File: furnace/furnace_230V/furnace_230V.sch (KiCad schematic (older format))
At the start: 3 parts

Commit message: Add files via upload
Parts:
- removed J?: CWF-4R, symbol Connector_Generic:Conn_01x04
- added J3: IDC-6, Connector_IDC:IDC-Header_2x03_P2.54mm_Vertical, symbol Connector_Generic:Conn_01x06
- J1, J2: renamed from J?; symbol Connector:Screw_Terminal_01x02 -> furnace_230V-rescue:Screw_Terminal_01x02-Connector
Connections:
- wire segments 81 -> 87
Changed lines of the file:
@@
 $EndDescr
 $Comp
-L Connector_Generic:Conn_01x04 J?
-U 1 1 60AAE60F
-P 10200 3200
-AR Path="/60AAC03E/60AAE60F" Ref="J?"  Part="1"
-AR Path="/60AAE60F" Ref="J?"  Part="1"
-F 0 "J?" H 10150 2800 50  0000 L CNN
-F 1 "CWF-4R" H 10050 2900 50  0000 L CNN
-F 2 "" H 10200 3200 50  0001 C CNN
-F 3 "~" H 10200 3200 50  0001 C CNN
-	1    10200 3200
-	1    0    0    1
-$EndComp
-$Comp
-L Connector:Screw_Terminal_01x02 J?
+L furnace_230V-rescue:Screw_Terminal_01x02-Connector J1
 U 1 1 60AAEFEC
 P 1800 1500
-F 0 "J?" H 1880 1492 50  0000 L CNN
+F 0 "J1" H 1880 1492 50  0000 L CNN
 F 1 "TC0" H 1880 1401 50  0000 L CNN
 F 2 "" H 1800 1500 50  0001 C CNN
@@
 $EndSheet
 $Comp
-L Connector:Screw_Terminal_01x02 J?
+L furnace_230V-rescue:Screw_Terminal_01x02-Connector J2
 U 1 1 60AB629C
 P 1800 2500
-F 0 "J?" H 1880 2492 50  0000 L CNN
+F 0 "J2" H 1880 2492 50  0000 L CNN
 F 1 "TC0" H 1880 2401 50  0000 L CNN
 F 2 "" H 1800 2500 50  0001 C CNN
@@
 Text Notes 6150 1050 2    197  ~ 0
 230V
-Text Notes 10500 3050 0    50   ~ 0
+Text Notes 10300 3000 0    50   ~ 0
 +5V
-Text Notes 10500 3350 0    50   ~ 0
+Text Notes 10300 3400 0    50   ~ 0
 GND
-Text Notes 10500 3150 0    50   ~ 0
+Text Notes 10300 3150 0    50   ~ 0
 UART_TX
-Text Notes 10500 3250 0    50   ~ 0
+Text Notes 10300 3250 0    50   ~ 0
 Heater
 Wire Wire Line
@@
 	9250 2400 8500 2400
 Wire Wire Line
-	10000 3000 9000 3000
+	10000 3000 9900 3000
 Connection ~ 9000 3000
 Wire Wire Line
 	9000 3000 9000 2100
 Wire Wire Line
-	10000 3300 9250 3300
+	10000 3300 9900 3300
 Connection ~ 9250 3300
 Wire Wire Line
@@
 Wire Wire Line
 	7300 5250 7500 5250
+$Comp
+L Connector_Generic:Conn_01x06 J3
+U 1 1 610690C6
+P 10200 3100
+F 0 "J3" H 10150 3550 50  0000 L CNN
+F 1 "IDC-6" H 10100 3450 50  0000 L CNN
+F 2 "Connector_IDC:IDC-Header_2x03_P2.54mm_Vertical" H 10200 3100 50  0001 C CNN
+F 3 "~" H 10200 3100 50  0001 C CNN
+	1    10200 3100
+	1    0    0    -1
+$EndComp
+Wire Wire Line
+	10000 2900 9900 2900
+Wire Wire Line
+	9900 2900 9900 3000
+Connection ~ 9900 3000
+Wire Wire Line
+	9900 3000 9000 3000
+Wire Wire Line
+	10000 3400 9900 3400
+Wire Wire Line
+	9900 3400 9900 3300
+Connection ~ 9900 3300
+Wire Wire Line
+	9900 3300 9250 3300
 $EndSCHEMATC

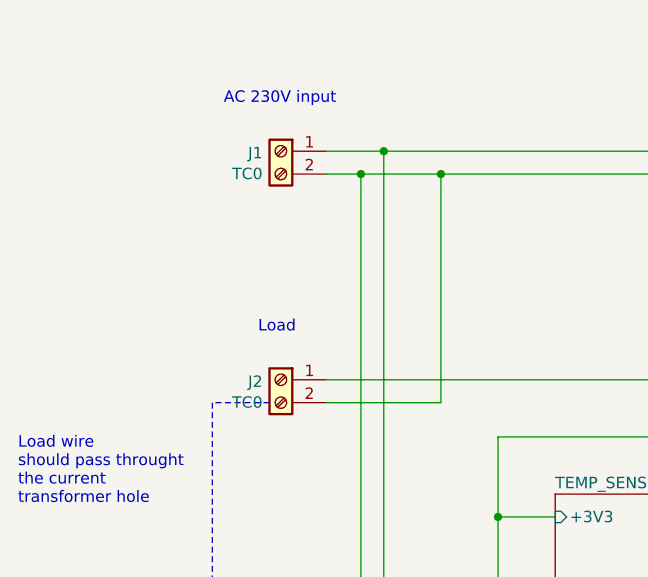
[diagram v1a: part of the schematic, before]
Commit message: Add files via upload
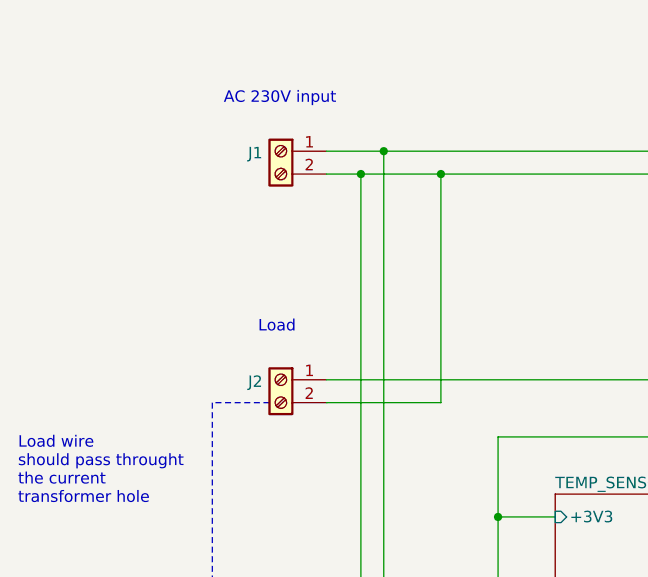
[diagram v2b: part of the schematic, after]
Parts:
- J1, J2: value TC0 -> (none)
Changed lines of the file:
@@
 P 1800 1500
 F 0 "J1" H 1880 1492 50  0000 L CNN
-F 1 "TC0" H 1880 1401 50  0000 L CNN
+F 1 " " H 1880 1401 50  0000 L CNN
 F 2 "" H 1800 1500 50  0001 C CNN
 F 3 "~" H 1800 1500 50  0001 C CNN
@@
 P 1800 2500
 F 0 "J2" H 1880 2492 50  0000 L CNN
-F 1 "TC0" H 1880 2401 50  0000 L CNN
+F 1 " " H 1880 2401 50  0000 L CNN
 F 2 "" H 1800 2500 50  0001 C CNN
 F 3 "~" H 1800 2500 50  0001 C CNN

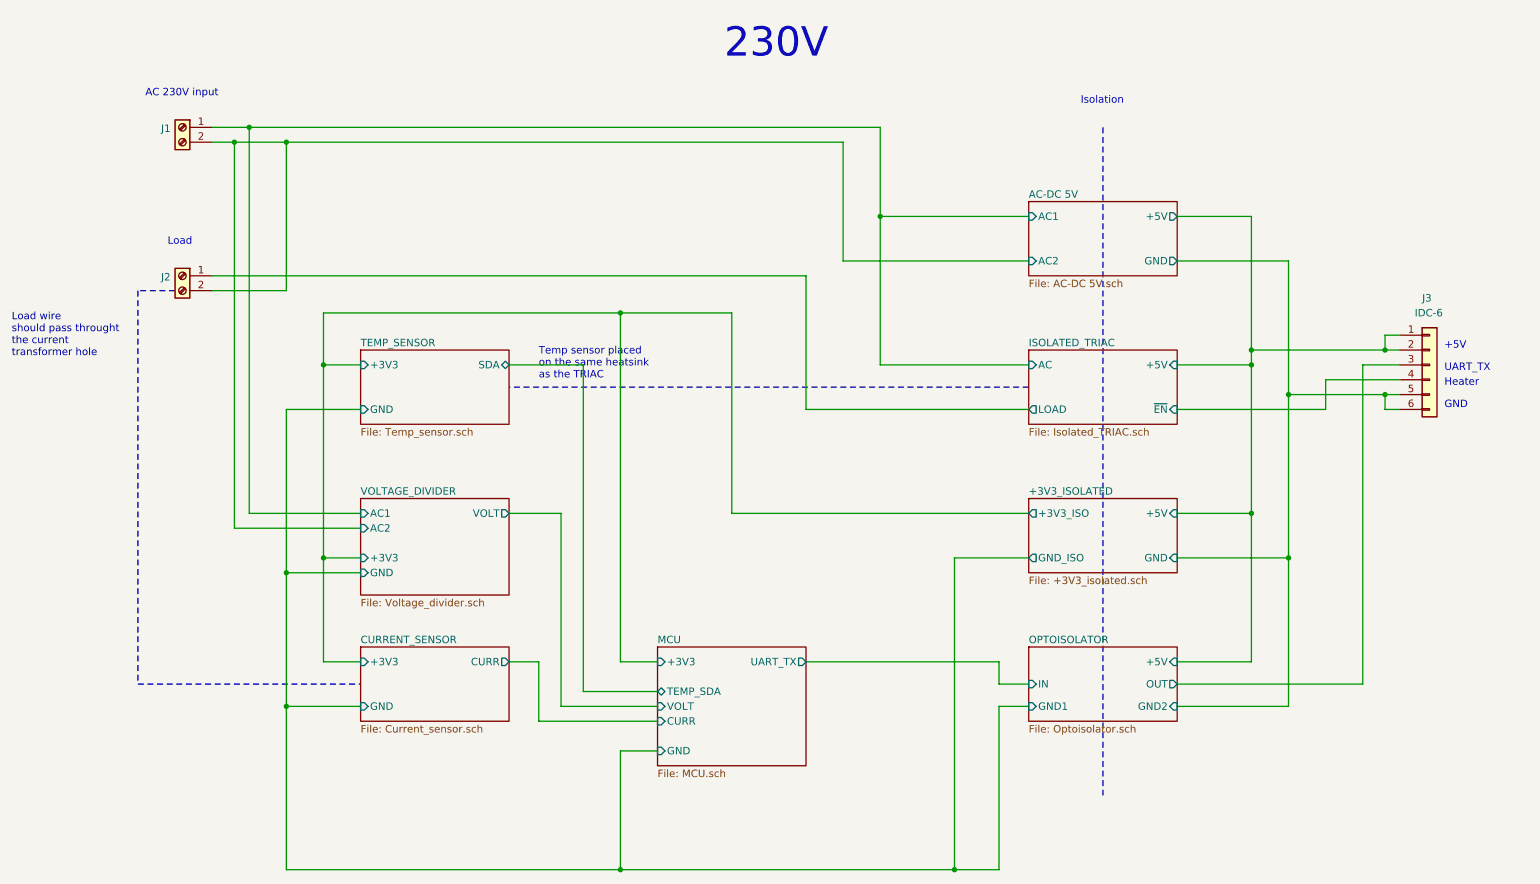
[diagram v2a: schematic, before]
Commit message: Add files via upload
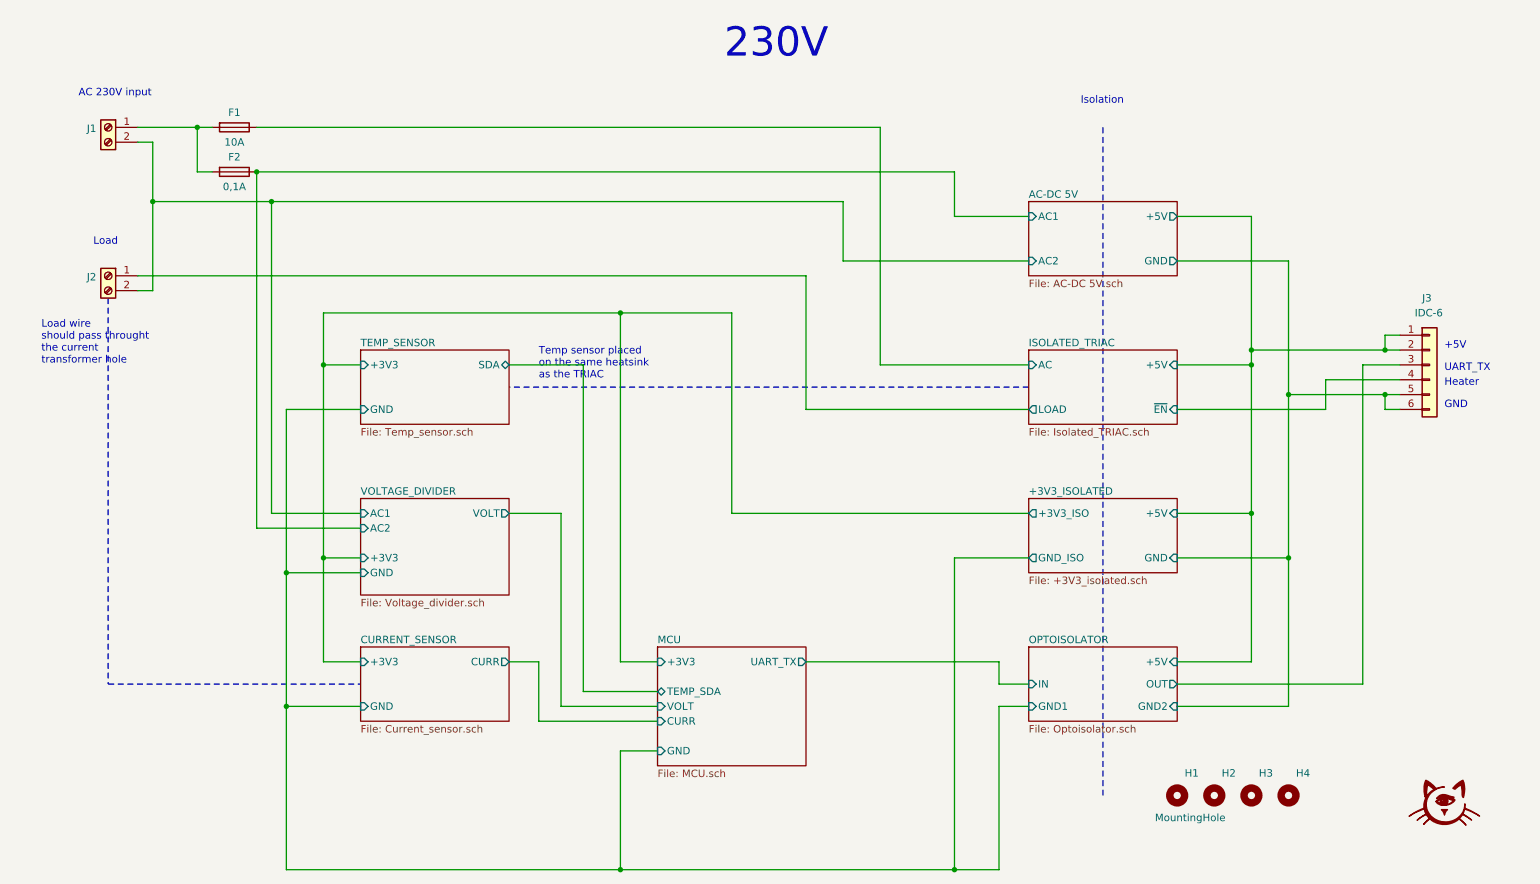
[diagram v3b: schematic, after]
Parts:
- added F1: 10A, Fuse:Fuseholder_Cylinder-5x20mm_Stelvio-Kontek_PTF78_Horizontal_Open, symbol furnace_230V-rescue:Fuse-Device
- added F2: 0,1A, Fuse:Fuseholder_Cylinder-5x20mm_Stelvio-Kontek_PTF78_Horizontal_Open, symbol furnace_230V-rescue:Fuse-Device
- added G1: LOGO, furnace_230V:stamp, symbol stamp:LOGO
- added H1, H2, H3, H4: MountingHole, furnace_230V:hole_D3.5mm, symbol Mechanical:MountingHole
- J1, J2: footprint (none) -> furnace_230V:KF7.62-2P
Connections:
- net AC-DC 5V/AC1: now also F2.1; no longer J1.1 (Pin_1)
- new net: F1.2, F2.2, J1.1 (Pin_1)
- new net ISOLATED_TRIAC/AC: F1.1
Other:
- moved on the sheet: J1, J2
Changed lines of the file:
@@
 L furnace_230V-rescue:Screw_Terminal_01x02-Connector J1
 U 1 1 60AAEFEC
-P 1800 1500
-F 0 "J1" H 1880 1492 50  0000 L CNN
-F 1 " " H 1880 1401 50  0000 L CNN
-F 2 "" H 1800 1500 50  0001 C CNN
-F 3 "~" H 1800 1500 50  0001 C CNN
-	1    1800 1500
+P 1300 1500
+F 0 "J1" H 1380 1492 50  0000 L CNN
+F 1 " " H 1380 1401 50  0000 L CNN
+F 2 "furnace_230V:KF7.62-2P" H 1300 1500 50  0001 C CNN
+F 3 "~" H 1300 1500 50  0001 C CNN
+	1    1300 1500
 	-1   0    0    -1
 $EndComp
@@
 L furnace_230V-rescue:Screw_Terminal_01x02-Connector J2
 U 1 1 60AB629C
-P 1800 2500
-F 0 "J2" H 1880 2492 50  0000 L CNN
-F 1 " " H 1880 2401 50  0000 L CNN
-F 2 "" H 1800 2500 50  0001 C CNN
-F 3 "~" H 1800 2500 50  0001 C CNN
-	1    1800 2500
+P 1300 2500
+F 0 "J2" H 1380 2492 50  0000 L CNN
+F 1 " " H 1380 2401 50  0000 L CNN
+F 2 "furnace_230V:KF7.62-2P" H 1300 2500 50  0001 C CNN
+F 3 "~" H 1300 2500 50  0001 C CNN
+	1    1300 2500
 	-1   0    0    -1
 $EndComp
@@
 F4 "GND" I L 3000 5400 50
 $EndSheet
-Text Notes 1550 1300 0    50   ~ 0
+Text Notes 1100 1300 0    50   ~ 0
 AC 230V input
 Wire Notes Line rgb(255, 0, 0)
 	8000 1500 8000 6000
 Wire Notes Line
-	1750 2600 1500 2600
+	1300 2650 1300 5250
 Wire Notes Line
-	1500 2600 1500 5250
-Wire Notes Line
-	1500 5250 3000 5250
+	1300 5250 3000 5250
 Wire Notes Line
 	7500 3250 4000 3250
 Text Notes 7850 1350 0    50   ~ 0
 Isolation
-Text Notes 650  3050 0    50   ~ 0
+Text Notes 850  3100 0    50   ~ 0
 Load wire \nshould pass throught\nthe current \ntransformer hole
 Text Notes 4200 3200 0    50   ~ 0
 Temp sensor placed \non the same heatsink\nas the TRIAC
-Text Notes 1700 2300 0    50   ~ 0
+Text Notes 1200 2300 0    50   ~ 0
 Load
 Wire Wire Line
-	6500 1500 6500 2100
-Wire Wire Line
-	6500 2100 7500 2100
-Wire Wire Line
 	7500 3100 6500 3100
 Wire Wire Line
-	6500 3100 6500 2100
-Connection ~ 6500 2100
-Wire Wire Line
 	7500 3400 6000 3400
 Wire Wire Line
 	7500 2400 6250 2400
 Wire Wire Line
-	6250 2400 6250 1600
-Wire Wire Line
-	2000 1500 2250 1500
-Wire Wire Line
-	2000 1600 2150 1600
+	6250 2400 6250 2000
 Wire Wire Line
 	6000 3400 6000 2500
-Wire Wire Line
-	6000 2500 2000 2500
-Wire Wire Line
-	2000 2600 2500 2600
-Wire Wire Line
-	2500 2600 2500 1600
-Connection ~ 2500 1600
-Wire Wire Line
-	2500 1600 6250 1600
 Text Notes 6150 1050 2    197  ~ 0
 230V
@@
 	2500 5400 2500 4500
 Wire Wire Line
-	3000 4100 2250 4100
-Wire Wire Line
-	2250 4100 2250 1500
-Connection ~ 2250 1500
-Wire Wire Line
-	2250 1500 6500 1500
-Wire Wire Line
-	3000 4200 2150 4200
-Wire Wire Line
-	2150 4200 2150 1600
-Connection ~ 2150 1600
-Wire Wire Line
-	2150 1600 2500 1600
+	3000 4100 2400 4100
+Wire Wire Line
+	2400 4100 2400 2000
+Wire Wire Line
+	3000 4200 2300 4200
+Wire Wire Line
+	2300 4200 2300 1800
 Wire Wire Line
 	5000 5700 4750 5700
@@
 Wire Wire Line
 	9900 3300 9250 3300
+$Comp
+L stamp:LOGO G1
+U 1 1 610EDF1B
+P 10300 6050
+F 0 "G1" H 10300 5928 60  0001 C CNN
+F 1 "LOGO" H 10300 6172 60  0001 C CNN
+F 2 "furnace_230V:stamp" H 10300 6050 50  0001 C CNN
+F 3 "" H 10300 6050 50  0001 C CNN
+	1    10300 6050
+	1    0    0    -1
+$EndComp
+$Comp
+L Mechanical:MountingHole H1
+U 1 1 6110929D
+P 8500 6000
+F 0 "H1" H 8550 6150 50  0000 L CNN
+F 1 "MountingHole" H 8350 5850 50  0000 L CNN
+F 2 "furnace_230V:hole_D3.5mm" H 8500 6000 50  0001 C CNN
+F 3 "~" H 8500 6000 50  0001 C CNN
+	1    8500 6000
+	1    0    0    -1
+$EndComp
+$Comp
+L Mechanical:MountingHole H2
+U 1 1 6110B2E7
+P 8750 6000
+F 0 "H2" H 8800 6150 50  0000 L CNN
+F 1 "MountingHole" H 8600 5850 50  0001 L CNN
+F 2 "furnace_230V:hole_D3.5mm" H 8750 6000 50  0001 C CNN
+F 3 "~" H 8750 6000 50  0001 C CNN
+	1    8750 6000
+	1    0    0    -1
+$EndComp
+$Comp
+L Mechanical:MountingHole H3
+U 1 1 6110B4DC
+P 9000 6000
+F 0 "H3" H 9050 6150 50  0000 L CNN
+F 1 "MountingHole" H 8850 5850 50  0001 L CNN
+F 2 "furnace_230V:hole_D3.5mm" H 9000 6000 50  0001 C CNN
+F 3 "~" H 9000 6000 50  0001 C CNN
+	1    9000 6000
+	1    0    0    -1
+$EndComp
+$Comp
+L Mechanical:MountingHole H4
+U 1 1 6110B613
+P 9250 6000
+F 0 "H4" H 9300 6150 50  0000 L CNN
+F 1 "MountingHole" H 9100 5850 50  0001 L CNN
+F 2 "furnace_230V:hole_D3.5mm" H 9250 6000 50  0001 C CNN
+F 3 "~" H 9250 6000 50  0001 C CNN
+	1    9250 6000
+	1    0    0    -1
+$EndComp
+$Comp
+L furnace_230V-rescue:Fuse-Device F?
+U 1 1 61103E7E
+P 2150 1800
+AR Path="/60AABABA/61103E7E" Ref="F?"  Part="1"
+AR Path="/61103E7E" Ref="F2"  Part="1"
+F 0 "F2" V 2050 1800 50  0000 C CNN
+F 1 "0,1A" V 2250 1800 50  0000 C CNN
+F 2 "Fuse:Fuseholder_Cylinder-5x20mm_Stelvio-Kontek_PTF78_Horizontal_Open" V 2080 1800 50  0001 C CNN
+F 3 "~" H 2150 1800 50  0001 C CNN
+	1    2150 1800
+	0    1    1    0
+$EndComp
+$Comp
+L furnace_230V-rescue:Fuse-Device F?
+U 1 1 61107140
+P 2150 1500
+AR Path="/60AAE0B8/61107140" Ref="F?"  Part="1"
+AR Path="/61107140" Ref="F1"  Part="1"
+F 0 "F1" V 2050 1500 50  0000 C CNN
+F 1 "10A" V 2250 1500 50  0000 C CNN
+F 2 "Fuse:Fuseholder_Cylinder-5x20mm_Stelvio-Kontek_PTF78_Horizontal_Open" V 2080 1500 50  0001 C CNN
+F 3 "~" H 2150 1500 50  0001 C CNN
+	1    2150 1500
+	0    1    1    0
+$EndComp
+Wire Wire Line
+	6500 1500 6500 3100
+Wire Wire Line
+	1600 2600 1600 2000
+Wire Wire Line
+	1600 1600 1500 1600
+Wire Wire Line
+	6250 2000 2400 2000
+Connection ~ 1600 2000
+Wire Wire Line
+	1600 2000 1600 1600
+Connection ~ 2400 2000
+Wire Wire Line
+	2400 2000 1600 2000
+Wire Wire Line
+	1500 1500 1900 1500
+Wire Wire Line
+	2000 1800 1900 1800
+Wire Wire Line
+	1900 1800 1900 1500
+Connection ~ 1900 1500
+Wire Wire Line
+	1900 1500 2000 1500
+Wire Wire Line
+	2300 1500 6500 1500
+Wire Wire Line
+	2300 1800 7000 1800
+Wire Wire Line
+	7000 1800 7000 2100
+Wire Wire Line
+	7000 2100 7500 2100
+Connection ~ 2300 1800
+Wire Wire Line
+	1600 2600 1500 2600
+Wire Wire Line
+	1500 2500 6000 2500
 $EndSCHEMATC
